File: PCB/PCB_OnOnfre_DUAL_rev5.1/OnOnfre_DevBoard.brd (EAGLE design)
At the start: 44 x 41.7 mm, 30 parts, among them J1 9PIN 2.54MM, J3Y S8050, J7 8p, K1 PA1A-6VV, K2 PA1A-6VV, U2 esp12

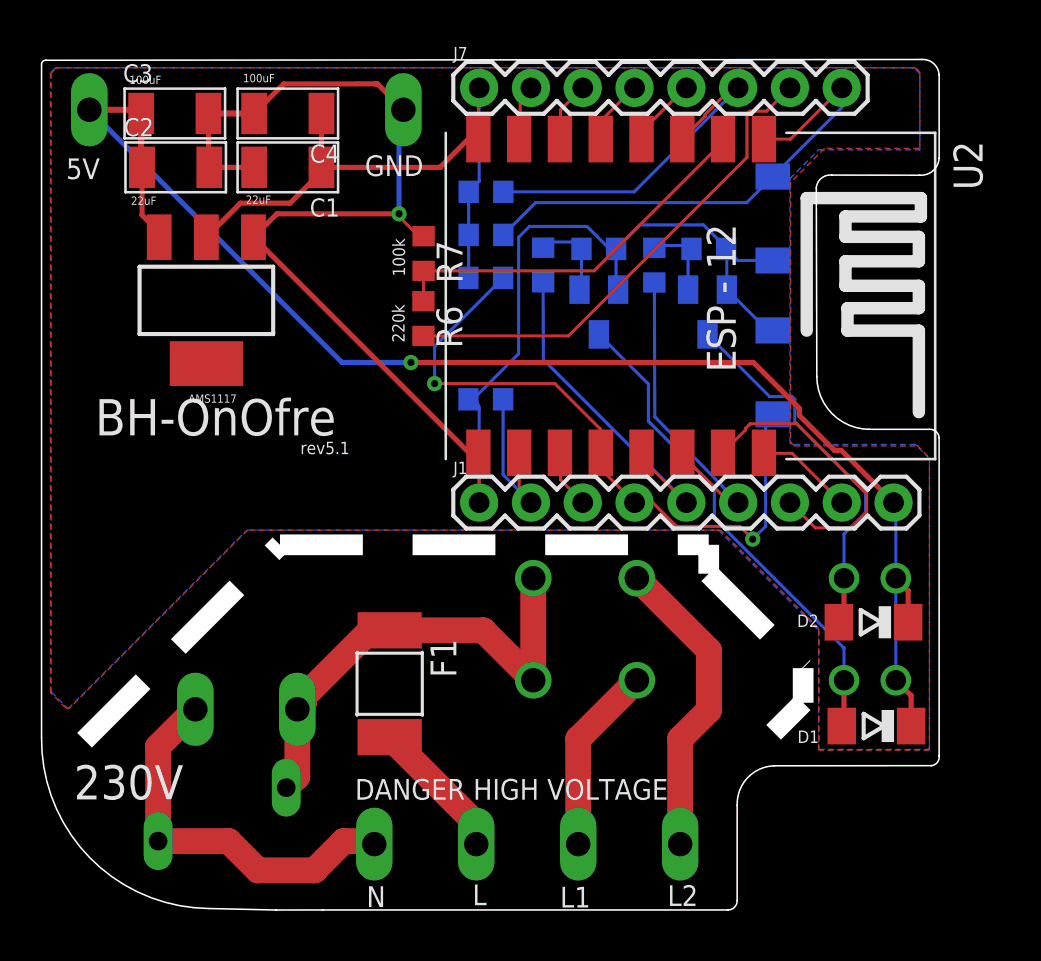
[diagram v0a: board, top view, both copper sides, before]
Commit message: board
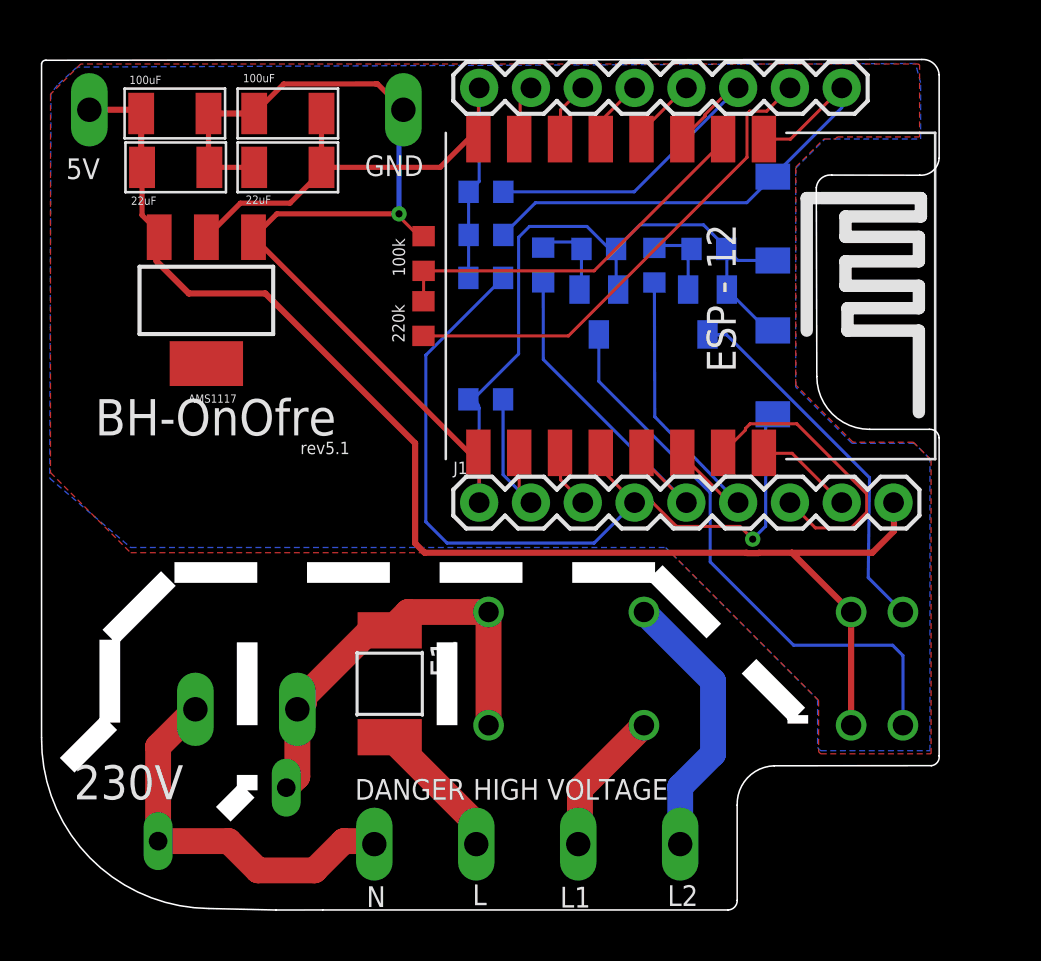
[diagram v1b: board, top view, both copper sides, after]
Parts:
- removed D1, D2: 1N4148, diode:SOD80C
- K1, K2: value PA1A-6VV -> OMRON-G3MB-202P-SSR2; device relay:PA -> Omron G3MB 202p SSR:OMRON-G3MB-202P-SSR
- moved K1 1.84 mm to (35.3, 13.7), turned to 180 degrees
- moved K2 1.65 mm to (35.3, 19.3), turned to 180 degrees
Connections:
- net LINE_L: now also K1.1, K2.1; no longer K1.COM, K2.COM
- net LINE_ONE_OUT: now also K1.2; no longer K1.NO
- net LINE_TWO_OUT: now also K2.2; no longer K2.NO
- net N$1: now also K1.4; no longer D1.A, K1.2
- net N$9: now also K2.4; no longer D2.A, K2.2
- net VCC: now also K1.3, K2.3; no longer D1.C, D2.C, K1.1, K2.1
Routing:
- net GPIO0: track 33.6 -> 41.4 mm, vias 2 -> 1
- net N$1: track 24.2 -> 28.2 mm
- net VCC: track 71.0 -> 67.4 mm, vias 1 -> 0
- net LINE_L: track 23.4 -> 21.1 mm
- net LINE_ONE_OUT: track 9.23 -> 7.16 mm
- net LINE_TWO_OUT: track 15.1 -> 13.5 mm
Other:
- outline, holes or cut-outs redrawn
